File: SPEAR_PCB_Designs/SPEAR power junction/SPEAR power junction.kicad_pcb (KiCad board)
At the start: 2 copper layers, 77 x 46.5 mm, 7 parts, among them J1 XT30PW-M, J2 XT30PW-M, J3 XT30PW-M, J5 XT90PW-M

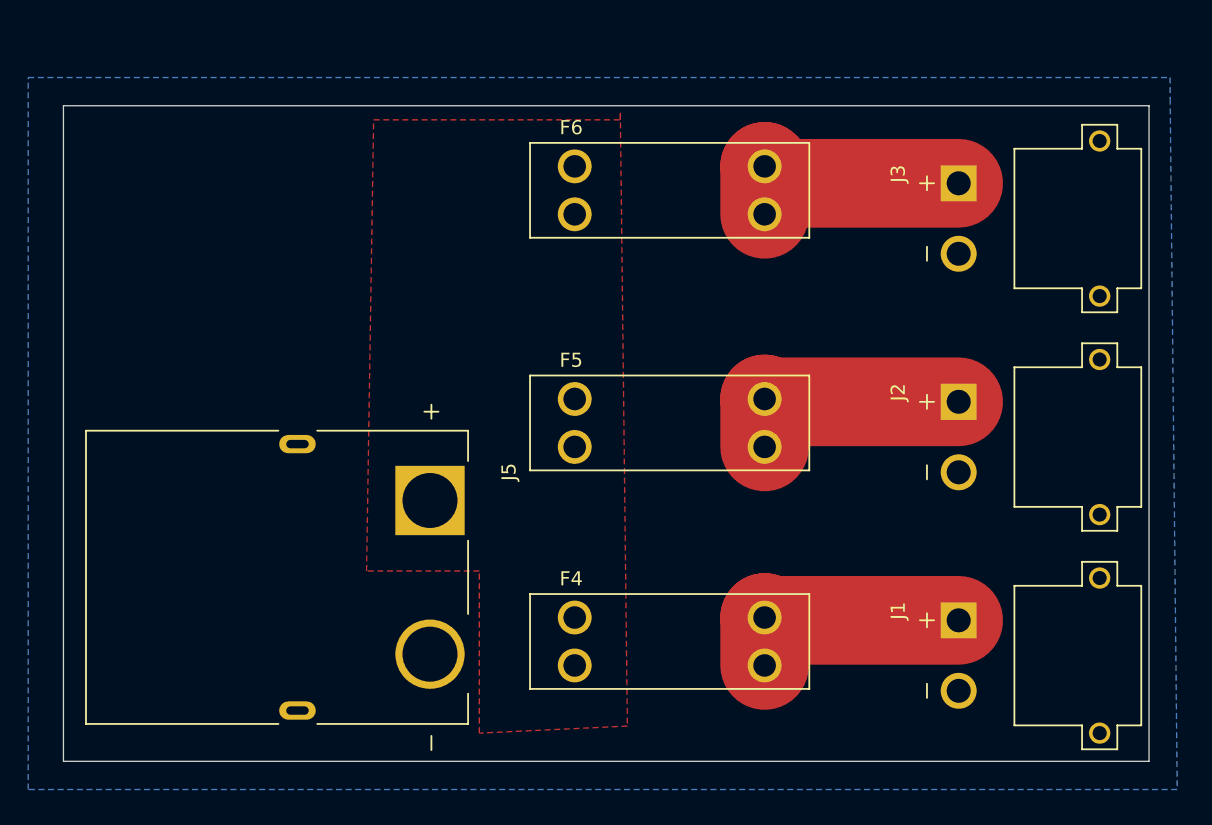
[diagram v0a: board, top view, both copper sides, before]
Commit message: Updated Power junction design and fabrication folder
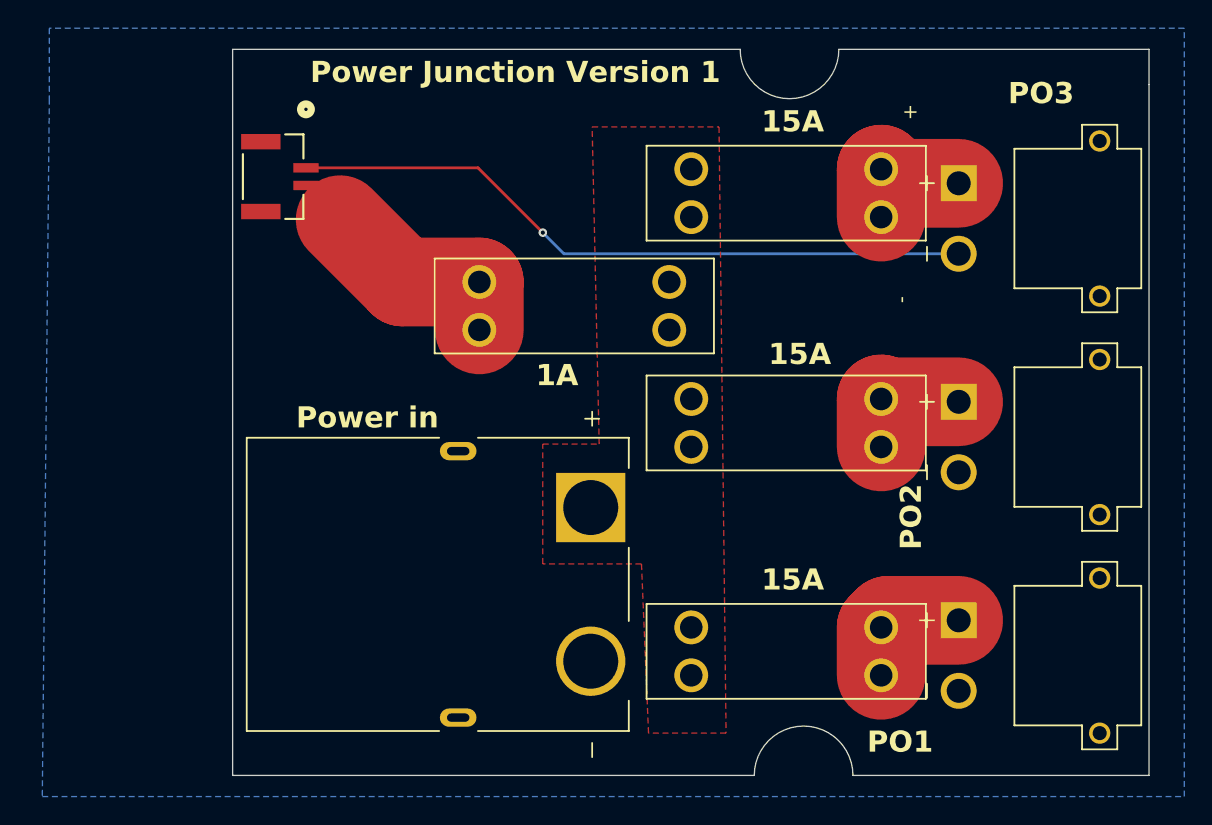
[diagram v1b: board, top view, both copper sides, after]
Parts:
- added F1: 3557-15, 3557-15:FUSE_3557-15, F.Cu at (157.2, 81.7)
- added J4: SM02B-GHS-TB, SM02B-GHS-TB:CONN_SM02B-GHS_JST, F.Cu at (135.9, 72.5)
- moved J5 11.4 mm to (149.0, 101.5)
- moved F4 8.29 mm to (172.3, 106.2)
- moved F6 8.27 mm to (172.3, 73.7)
- moved F5 8.26 mm to (172.3, 90.0)
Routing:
- net GND: track 0.00 -> 48.8 mm, vias 0 -> 1
- net Net-(F1-Pad2_1): track 0.00 -> 15.1 mm
- net Net-(F6-Pad2_1): track 17.7 -> 9.31 mm
- net Net-(F5-Pad2_1): track 17.2 -> 8.98 mm
- net Net-(F4-Pad2_1): track 17.2 -> 9.11 mm
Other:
- board size 77 x 46.5 mm -> 65 x 51.5 mm
- board text added: "+"
- board text added: "-"
- board text added: "15A"
- board text added: "1A"
- board text added: "Joelle Adedun"
- board text added: "PO1"
- board text added: "PO2"
- board text added: "PO3"
- board text added: "Power Junction Version 1"
- board text added: "Power in"
- board text added: "SPEAR"
